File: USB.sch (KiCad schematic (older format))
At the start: 10 parts, among them P1 USB_OTG, P4 CONN_01X06, Q1 S8050, Q2 S8050, U2 CP2104

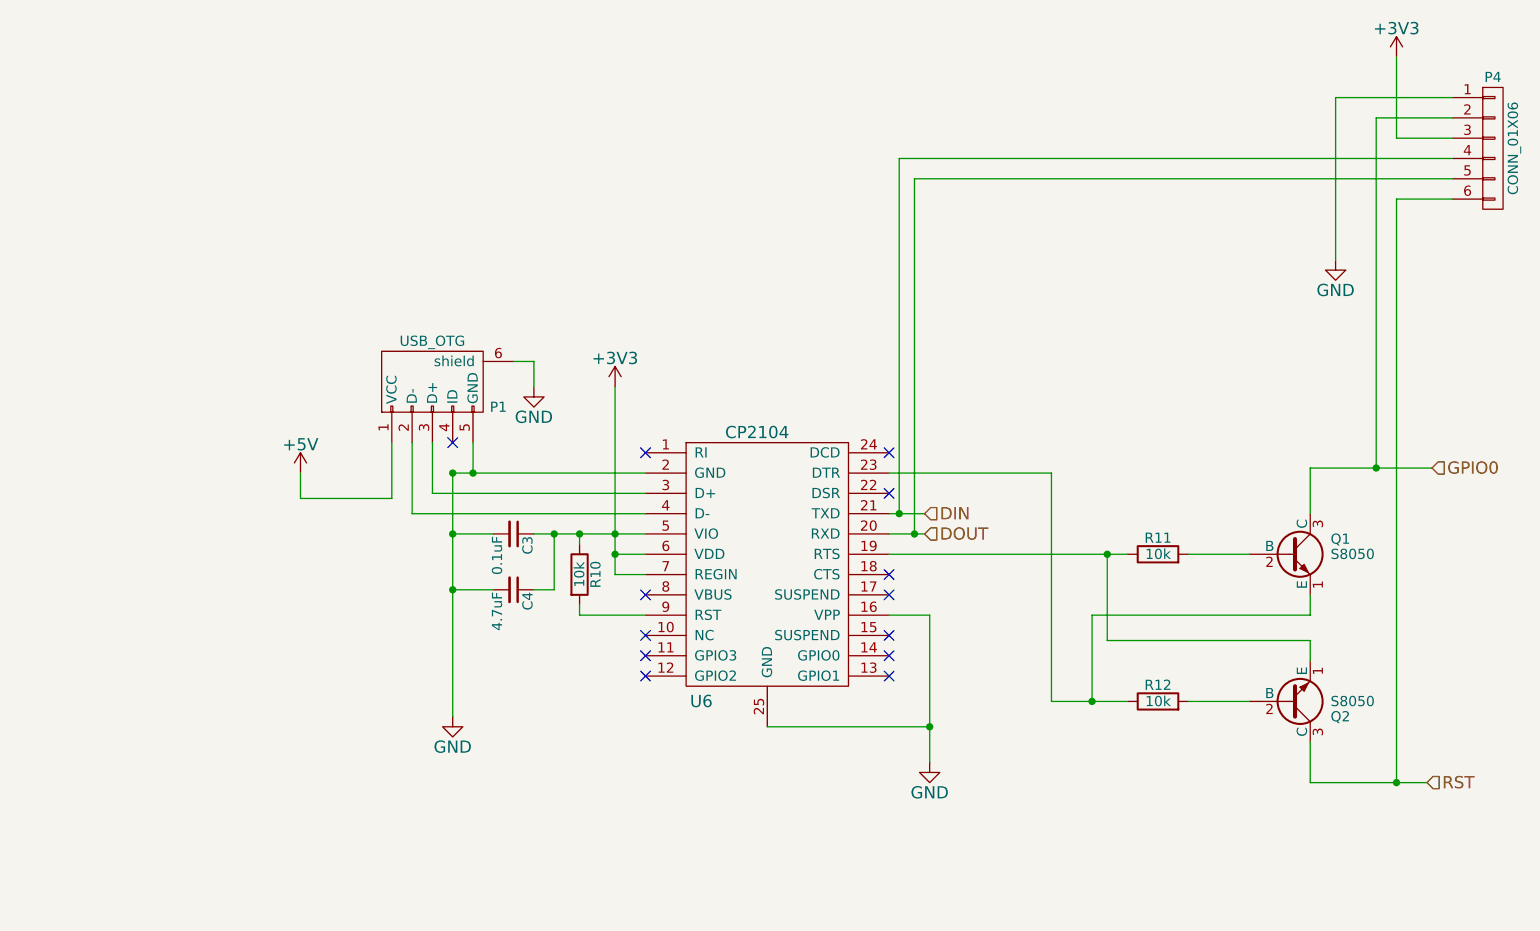
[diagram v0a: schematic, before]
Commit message: v3.2 of the PCB
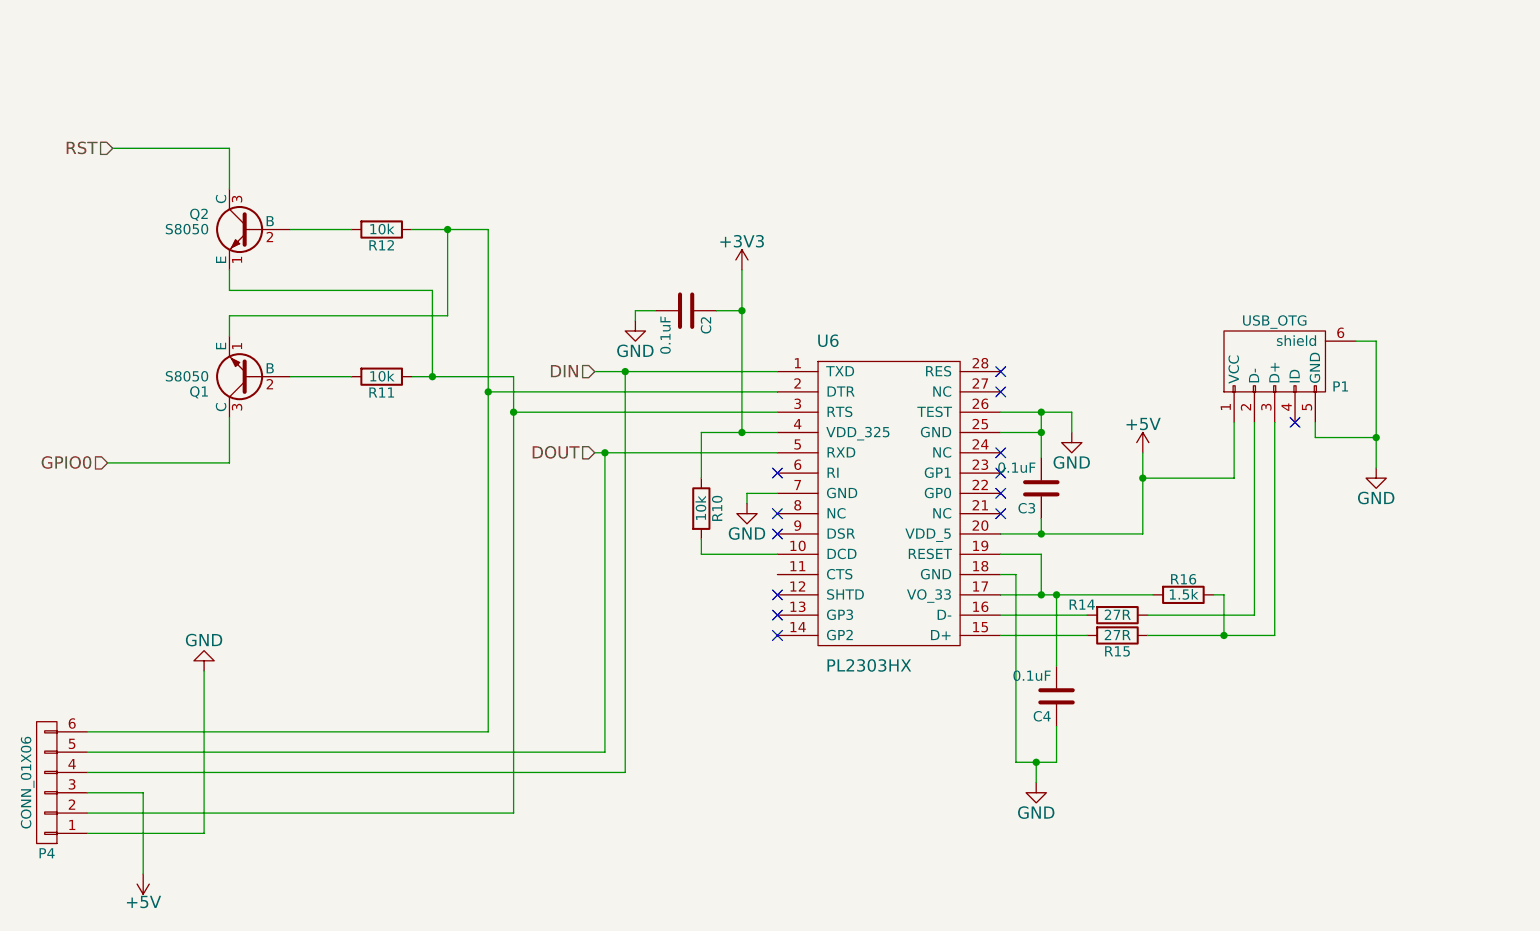
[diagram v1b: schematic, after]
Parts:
- removed C3: 0.1uF, Capacitors_SMD:C_0603, symbol C_Small
- removed C4: 4.7uF, Capacitors_SMD:C_0603, symbol C_Small
- removed U2: CP2104, Custom:QFN-24-1EP_4x4mm_Pitch0.5mm-easySolder, symbol CP2104
- added C2, C3, C4: 0.1uF, Capacitors_SMD:C_0603, symbol C
- added R14, R15: 27R, Resistors_SMD:R_0603, symbol R
- added R16: 1.5k, Resistors_SMD:R_0603, symbol R
- added U6: PL2303HX, Housings_SSOP:SSOP-28_5.3x10.2mm_Pitch0.65mm, symbol PL2303HX
- P4: footprint Pin_Headers:Pin_Header_Straight_1x06 -> Custom:6-PIN-EDGE-CONN
- R10: Description 0603 10k Resistor -> (none); Manufacturer Name (MFN) Generic -> (none); Package ID 0603 -> (none)
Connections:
- net +3V3: now also C2.1, U6.4 (VDD_325); no longer P4.3 (P3)
- net +5V: now also P4.3 (P3), C3.1, U6.20 (VDD_5)
- net DIN: now also U6.1 (TXD)
- net DOUT: now also U6.5 (RXD)
- net GND: now also C2.2, C3.2, C4.1, U6.18 (GND), U6.25 (GND), U6.26 (TEST), U6.7 (GND)
- net GPIO0: no longer P4.2 (P2)
- net RST: no longer P4.6 (P6)
- net at Q1.1 (E), R12.1: now also P4.6 (P6), U6.2 (DTR)
- net at Q2.1 (E), R11.1: now also P4.2 (P2), U6.3 (RTS)
- net at P1.3 (D+): now also R15.1, R16.1
- net at P1.2 (D-): now also R14.1
- net at R10.2: now also U6.10 (DCD)
- new net: R15.2, U6.15 (D+)
- new net: R14.2, U6.16 (D-)
- new net: C4.2, R16.2, U6.17 (VO_33), U6.19 (RESET)
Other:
- moved on the sheet: P1, P4, Q1, Q2, R11, R12

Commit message: v3.3 of the PCB
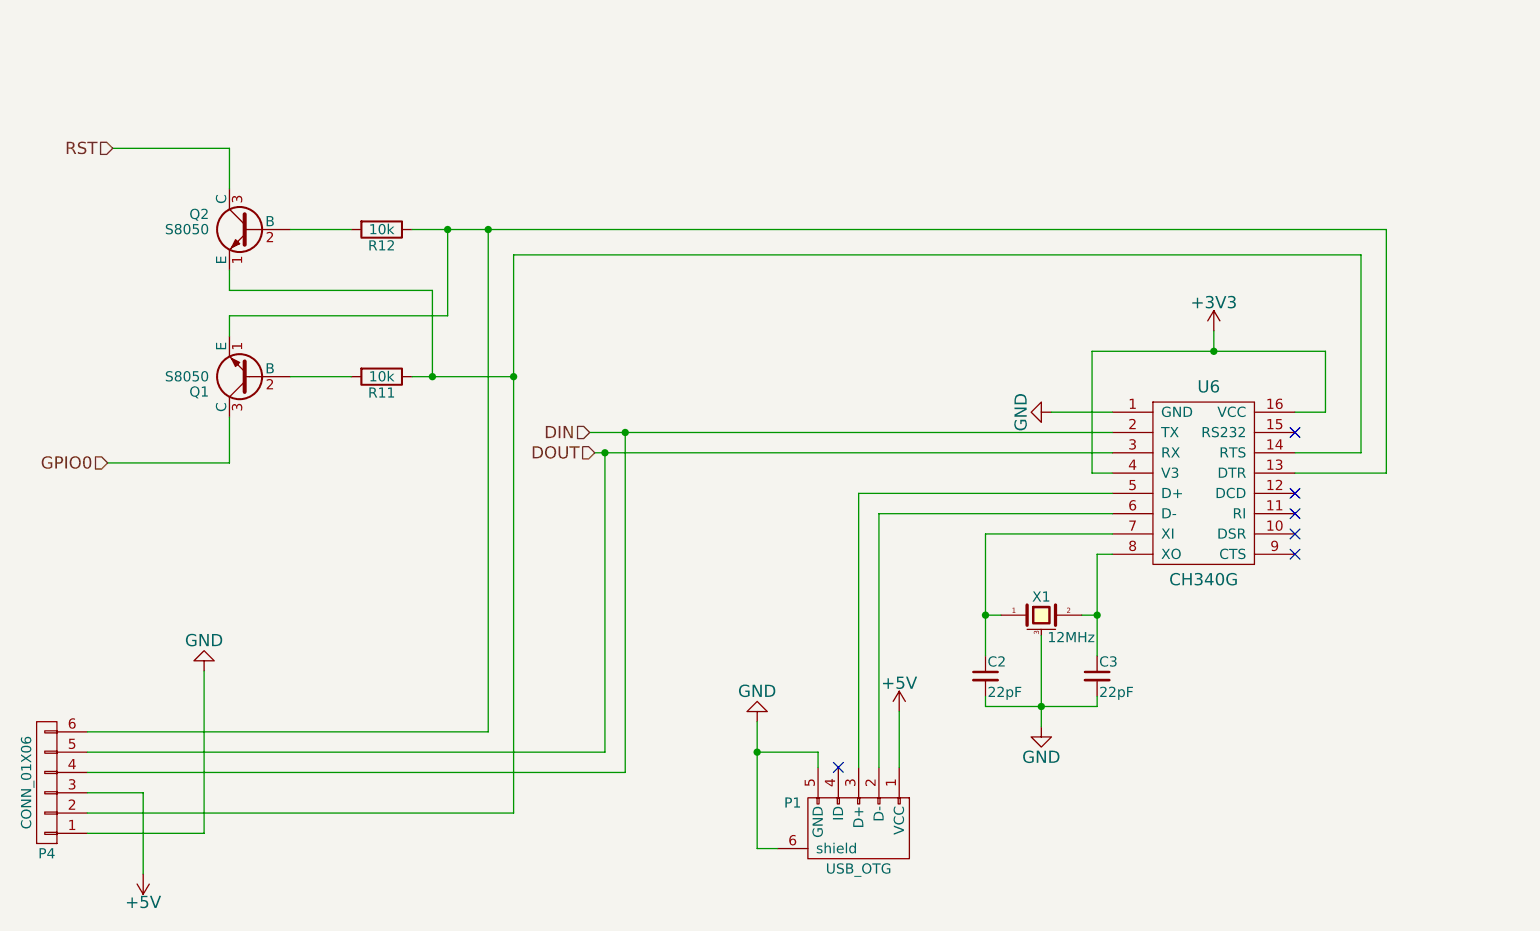
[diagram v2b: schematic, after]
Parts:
- removed C2, C3, C4: 0.1uF, Capacitors_SMD:C_0603, symbol C
- removed R10: 10k, Resistors_SMD:R_0603, symbol R
- removed R14, R15: 27R, Resistors_SMD:R_0603, symbol R
- removed R16: 1.5k, Resistors_SMD:R_0603, symbol R
- removed U6: PL2303HX, Housings_SSOP:SSOP-28_5.3x10.2mm_Pitch0.65mm, symbol PL2303HX
- added C2, C3: 22pF, Capacitors_SMD:C_0603, symbol C_Small
- added U6: CH340G, SMD_Packages:SO-16-N, symbol CH340G
- added X1: 12MHz, Crystals:crystal_FA238-TSX3225, symbol CRYSTAL_SMD
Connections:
- net +3V3: now also U6.16 (VCC), U6.4 (V3)
- net DIN: now also U6.2 (TX)
- net DOUT: now also U6.3 (RX)
- net GND: now also C2.2, C3.2, U6.1 (GND), X1.3 (case)
- net at P4.6 (P6), Q1.1 (E), R12.1: now also U6.13 (DTR)
- net at P4.2 (P2), Q2.1 (E), R11.1: now also U6.14 (RTS)
- net at P1.2 (D-): now also U6.6 (D-)
- net at P1.3 (D+): now also U6.5 (D+)
- new net: C2.1, U6.7 (XI), X1.1
- new net: C3.1, U6.8 (XO), X1.2
- no-connect marks 13 -> 6
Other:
- moved on the sheet: P1
